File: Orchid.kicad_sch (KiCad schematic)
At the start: 130 parts, among them J1 Battery_L, J2 Battery_R, SW1 SW_DPDT_x2, SW2 SW_DPDT_x2, U1 nice_nano, U2 nice_nano

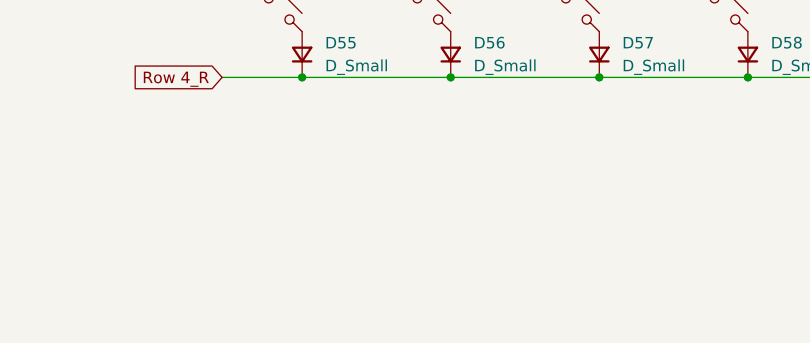
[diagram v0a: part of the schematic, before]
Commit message: Added title.
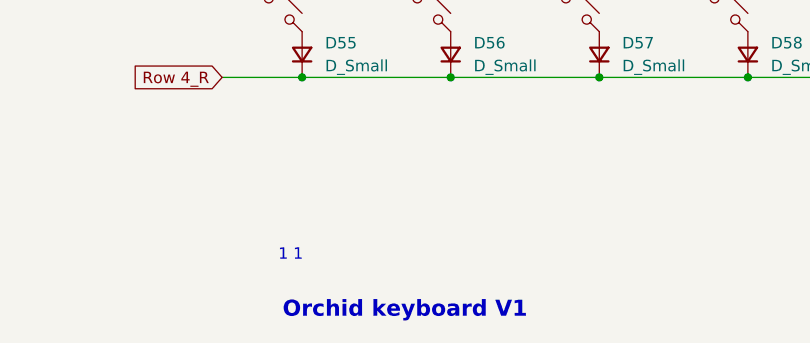
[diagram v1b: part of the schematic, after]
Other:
- note added: "1 1"
- note added: "Orchid keyboard V1"
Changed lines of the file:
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@@
+		)
+	)
+	(text "1 1"
+		(exclude_from_sim no)
+		(at 186.69 183.642 0)
+		(effects
+			(font
+				(size 1.27 1.27)
+			)
+		)
+	)
+	(text "Orchid keyboard V1\n"
+		(exclude_from_sim no)
+		(at 199.39 189.738 0)
+		(effects
+			(font
+				(size 1.778 1.778)
+				(thickness 0.3556)
+				(bold yes)
+			)
 		)
 	)
